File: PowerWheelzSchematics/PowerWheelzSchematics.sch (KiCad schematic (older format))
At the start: 0 parts

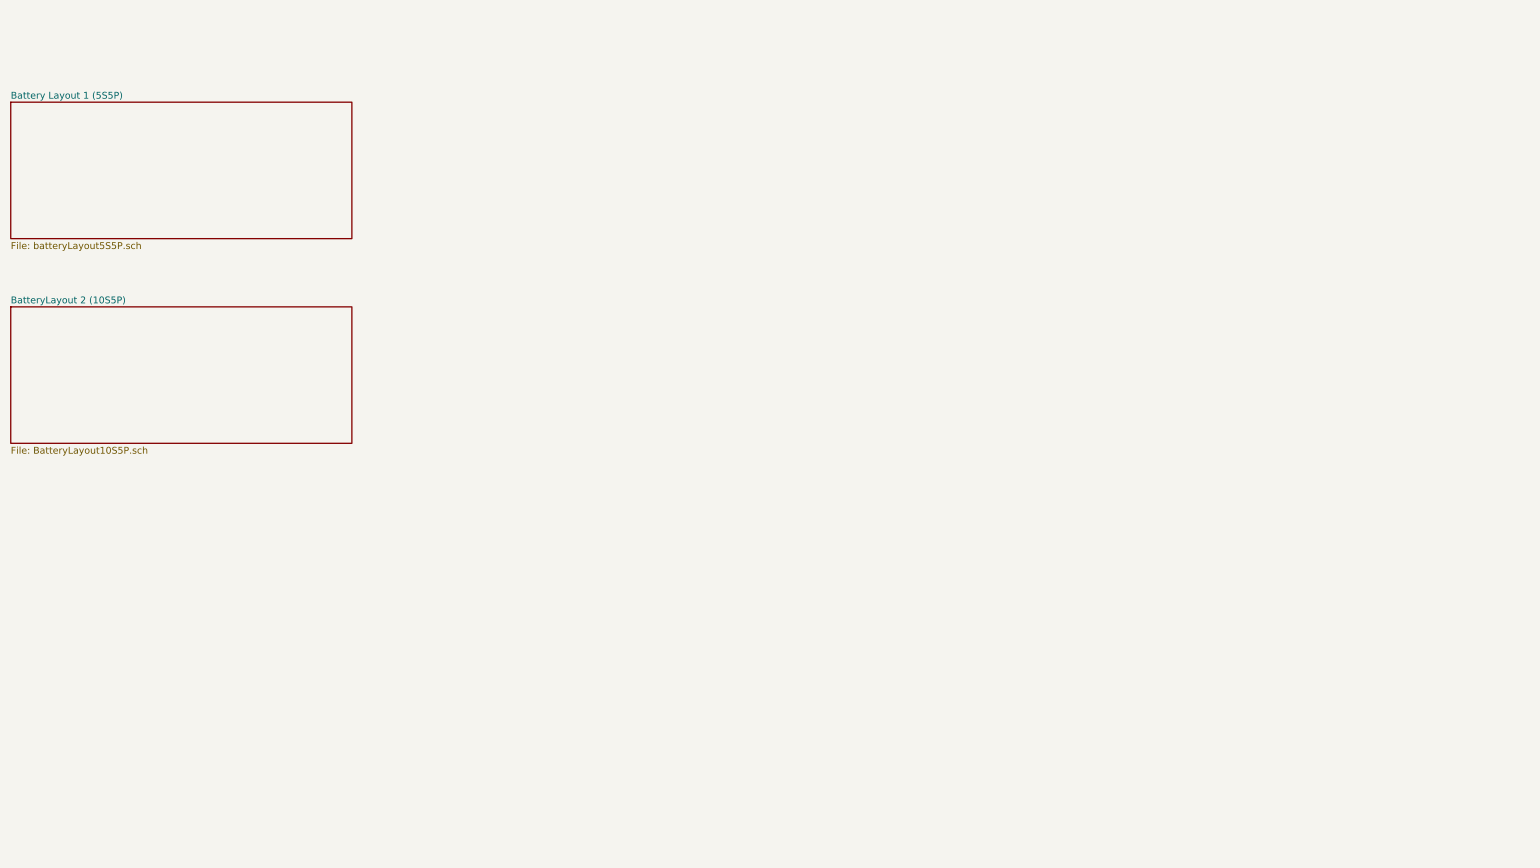
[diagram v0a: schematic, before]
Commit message: Big Update
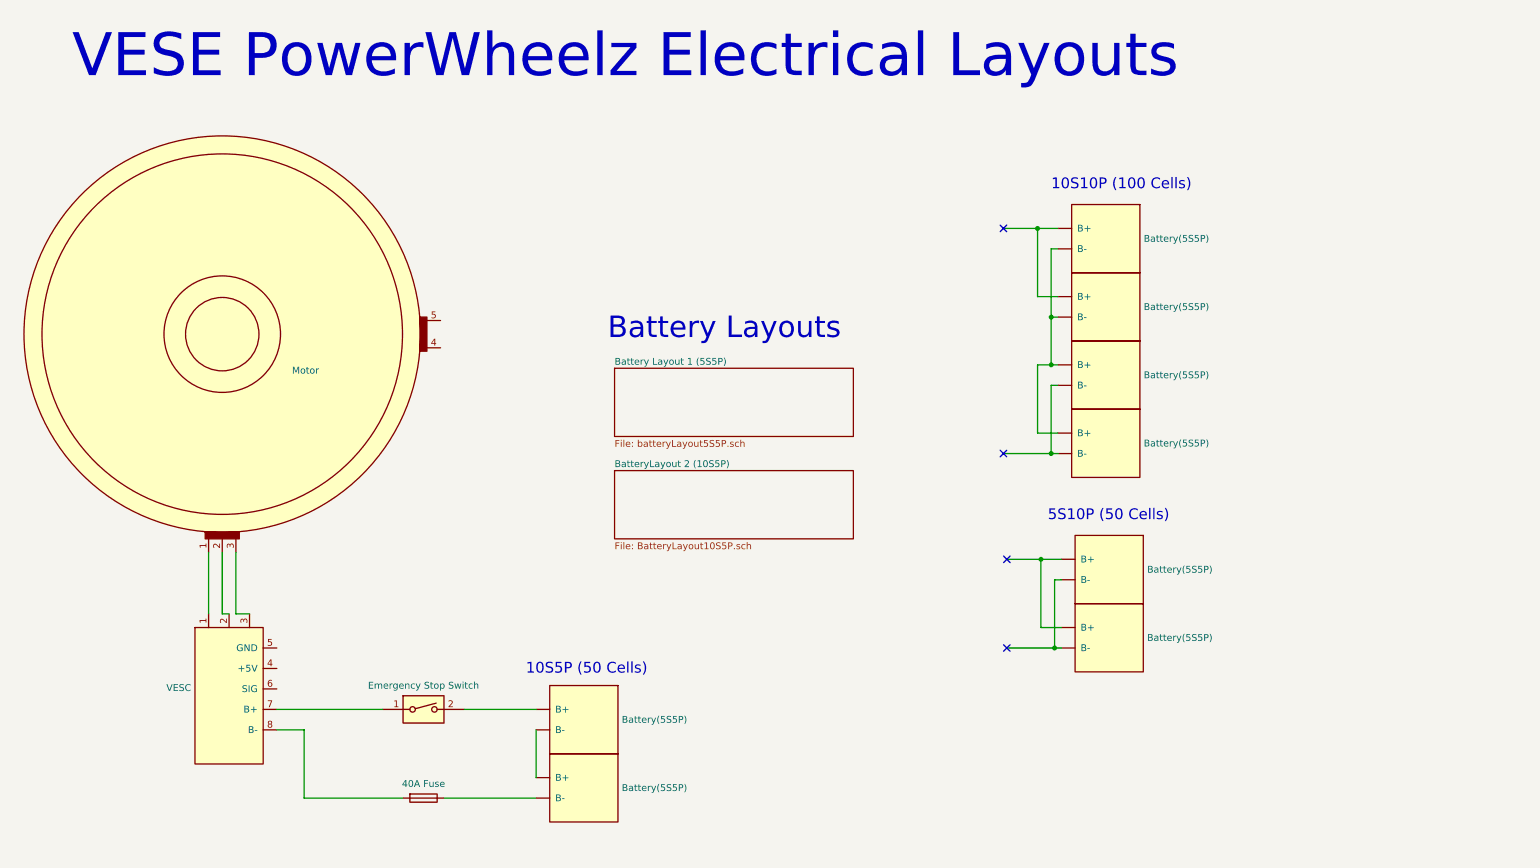
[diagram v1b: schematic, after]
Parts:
- added F: 40A Fuse, symbol Device:Fuse
- added SW?: Emergency Stop Switch, symbol Switch:SW_DIP_x01
- added U?: VESC, symbol VESE:VESC
- added U?: Motor, symbol VESE:Motor
- added U? (x8): Battery(5S5P), symbol VESE:Battery(5S5P)
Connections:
- new net: U?.1, U?.1
- new net: U?.2, U?.2
- new net: U?.3, U?.3
- new net: SW?.1, U?.7 (B+)
- new net: F.2, U?.8 (B-)
- new net: U?.~ (B-), U?.~ (B-) (x5)
- new net: U?.~ (B-), U?.~ (B-), U?.~ (B-), U?.~ (B-)
- new net: SW?.2, U?.~ (B-)
- new net: F.1, U?.~ (B-)
- no-connect marks 0 -> 4
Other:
- note added: "10S10P (100 Cells)"
- note added: "10S5P (50 Cells)"
- note added: "5S10P (50 Cells)"
- note added: "Battery Layouts"
- note added: "VESE PowerWheelz Electrical Layouts\n"
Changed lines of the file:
@@
 $EndDescr
 $Sheet
-S 1000 1250 2500 1000
+S 5425 3950 1750 500
+U 5FA8CE26
+F0 "BatteryLayout 2 (10S5P)" 50
+F1 "BatteryLayout10S5P.sch" 50
+$EndSheet
+Wire Wire Line
+	2600 5000 2550 5000
+Wire Wire Line
+	2650 5000 2750 5000
+$Comp
+L VESE:Motor U?
+U 1 1 5F97A74D
+P 2550 2950
+F 0 "U?" H 2550 2950 50  0001 C CNN
+F 1 "Motor" H 3061 2684 50  0000 L CNN
+F 2 "" H 2550 2950 50  0001 C CNN
+F 3 "" H 2550 2950 50  0001 C CNN
+	1    2550 2950
+	1    0    0    -1
+$EndComp
+$Comp
+L VESE:Battery(5S5P) U?
+U 1 1 5F985BDF
+P 9275 3000
+F 0 "U?" H 9275 3000 50  0001 C CNN
+F 1 "Battery(5S5P)" V 9525 3028 50  0000 L CNN
+F 2 "" H 9275 3000 50  0001 C CNN
+F 3 "" H 9275 3000 50  0001 C CNN
+	1    9275 3000
+	0    1    1    0
+$EndComp
+$Comp
+L VESE:Battery(5S5P) U?
+U 1 1 5F987B8F
+P 9275 3500
+F 0 "U?" H 9275 3500 50  0001 C CNN
+F 1 "Battery(5S5P)" V 9525 3528 50  0000 L CNN
+F 2 "" H 9275 3500 50  0001 C CNN
+F 3 "" H 9275 3500 50  0001 C CNN
+	1    9275 3500
+	0    1    1    0
+$EndComp
+Wire Wire Line
+	4850 5850 4850 6200
+Wire Wire Line
+	3150 5850 2950 5850
+Wire Wire Line
+	3150 6350 3150 5850
+$Comp
+L VESE:VESC U?
+U 1 1 5F96E5B6
+P 2350 5100
+F 0 "U?" H 2350 5100 50  0001 C CNN
+F 1 "VESC" H 2322 4658 50  0000 R CNN
+F 2 "" H 2350 5100 50  0001 C CNN
+F 3 "" H 2350 5100 50  0001 C CNN
+	1    2350 5100
+	1    0    0    -1
+$EndComp
+$Comp
+L Switch:SW_DIP_x01 SW?
+U 1 1 5F9C224C
+P 4025 5700
+F 0 "SW?" H 4025 5967 50  0001 C CNN
+F 1 "Emergency Stop Switch" H 4025 5875 50  0000 C CNN
+F 2 "" H 4025 5700 50  0001 C CNN
+F 3 "~" H 4025 5700 50  0001 C CNN
+	1    4025 5700
+	1    0    0    -1
+$EndComp
+Wire Wire Line
+	3150 6350 3875 6350
+Wire Wire Line
+	2950 5700 3725 5700
+Wire Wire Line
+	4325 5700 4850 5700
+Text Notes 1450 1100 0    315  ~ 0
+VESE PowerWheelz Electrical Layouts\n
+Text Notes 5375 3000 0    157  ~ 0
+Battery Layouts
+$Sheet
+S 5425 3200 1750 500
 U 5F8680B4
 F0 "Battery Layout 1 (5S5P)" 50
 F1 "batteryLayout5S5P.sch" 50
 $EndSheet
-$Sheet
-S 1000 2750 2500 1000
-U 5FA8CE26
-F0 "BatteryLayout 2 (10S5P)" 50
-F1 "BatteryLayout10S5P.sch" 50
-$EndSheet
+Wire Wire Line
+	2450 4550 2450 5000
+Wire Wire Line
+	2550 4550 2550 5000
+Wire Wire Line
+	2650 4550 2650 5000
+$Comp
+L Device:Fuse F
+U 1 1 5F9D666D
+P 4025 6350
+F 0 "F" V 3828 6350 50  0001 C CNN
+F 1 "40A Fuse" V 3920 6350 50  0000 C CNN
+F 2 "" V 3955 6350 50  0001 C CNN
+F 3 "~" H 4025 6350 50  0001 C CNN
+	1    4025 6350
+	0    1    1    0
+$EndComp
+Wire Wire Line
+	4175 6350 4850 6350
+$Comp
+L VESE:Battery(5S5P) U?
+U 1 1 5F9E11C0
+P 9275 2000
+F 0 "U?" H 9275 2000 50  0001 C CNN
+F 1 "Battery(5S5P)" V 9525 2028 50  0000 L CNN
+F 2 "" H 9275 2000 50  0001 C CNN
+F 3 "" H 9275 2000 50  0001 C CNN
+	1    9275 2000
+	0    1    1    0
+$EndComp
+$Comp
+L VESE:Battery(5S5P) U?
+U 1 1 5F9E11C6
+P 9275 2500
+F 0 "U?" H 9275 2500 50  0001 C CNN
+F 1 "Battery(5S5P)" V 9525 2528 50  0000 L CNN
+F 2 "" H 9275 2500 50  0001 C CNN
+F 3 "" H 9275 2500 50  0001 C CNN
+	1    9275 2500
+	0    1    1    0
+$EndComp
+Wire Wire Line
+	8525 2675 8525 2175
+Wire Wire Line
+	8525 2175 8675 2175
+Wire Wire Line
+	8525 2675 8675 2675
+Wire Wire Line
+	8675 2325 8625 2325
+Wire Wire Line
+	8625 2325 8625 2825
+Wire Wire Line
+	8625 2825 8675 2825
+Wire Wire Line
+	8525 3175 8525 3675
+Wire Wire Line
+	8525 3675 8675 3675
+Wire Wire Line
+	8675 3325 8625 3325
+Wire Wire Line
+	8625 3325 8625 3825
+Wire Wire Line
+	8625 3825 8675 3825
+Wire Wire Line
+	8625 3825 8275 3825
+Connection ~ 8625 3825
+Wire Wire Line
+	8525 2175 8275 2175
+Connection ~ 8525 2175
+Wire Wire Line
+	8625 2825 8625 3175
+Wire Wire Line
+	8525 3175 8625 3175
+Connection ~ 8625 2825
+Connection ~ 8625 3175
+Wire Wire Line
+	8625 3175 8675 3175
+$Comp
+L VESE:Battery(5S5P) U?
+U 1 1 5F9F8610
+P 5450 5525
+F 0 "U?" H 5450 5525 50  0001 C CNN
+F 1 "Battery(5S5P)" V 5700 5553 50  0000 L CNN
+F 2 "" H 5450 5525 50  0001 C CNN
+F 3 "" H 5450 5525 50  0001 C CNN
+	1    5450 5525
+	0    1    1    0
+$EndComp
+$Comp
+L VESE:Battery(5S5P) U?
+U 1 1 5F9F8616
+P 5450 6025
+F 0 "U?" H 5450 6025 50  0001 C CNN
+F 1 "Battery(5S5P)" V 5700 6053 50  0000 L CNN
+F 2 "" H 5450 6025 50  0001 C CNN
+F 3 "" H 5450 6025 50  0001 C CNN
+	1    5450 6025
+	0    1    1    0
+$EndComp
+NoConn ~ 8275 3825
+NoConn ~ 8275 2175
+Text Notes 4775 5450 0    79   ~ 0
+10S5P (50 Cells)
+Text Notes 8625 1900 0    79   ~ 0
+10S10P (100 Cells)
+$Comp
+L VESE:Battery(5S5P) U?
+U 1 1 5FA0FAAC
+P 9300 4425
+F 0 "U?" H 9300 4425 50  0001 C CNN
+F 1 "Battery(5S5P)" V 9550 4453 50  0000 L CNN
+F 2 "" H 9300 4425 50  0001 C CNN
+F 3 "" H 9300 4425 50  0001 C CNN
+	1    9300 4425
+	0    1    1    0
+$EndComp
+$Comp
+L VESE:Battery(5S5P) U?
+U 1 1 5FA0FAB2
+P 9300 4925
+F 0 "U?" H 9300 4925 50  0001 C CNN
+F 1 "Battery(5S5P)" V 9550 4953 50  0000 L CNN
+F 2 "" H 9300 4925 50  0001 C CNN
+F 3 "" H 9300 4925 50  0001 C CNN
+	1    9300 4925
+	0    1    1    0
+$EndComp
+Wire Wire Line
+	8700 5100 8550 5100
+Wire Wire Line
+	8550 5100 8550 4600
+Wire Wire Line
+	8550 4600 8700 4600
+Wire Wire Line
+	8700 4750 8650 4750
+Wire Wire Line
+	8650 4750 8650 5250
+Wire Wire Line
+	8650 5250 8700 5250
+Wire Wire Line
+	8550 4600 8300 4600
+Connection ~ 8550 4600
+Wire Wire Line
+	8650 5250 8300 5250
+Connection ~ 8650 5250
+NoConn ~ 8300 4600
+NoConn ~ 8300 5250
+Text Notes 8600 4325 0    79   ~ 0
+5S10P (50 Cells)
 $EndSCHEMATC

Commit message: supply
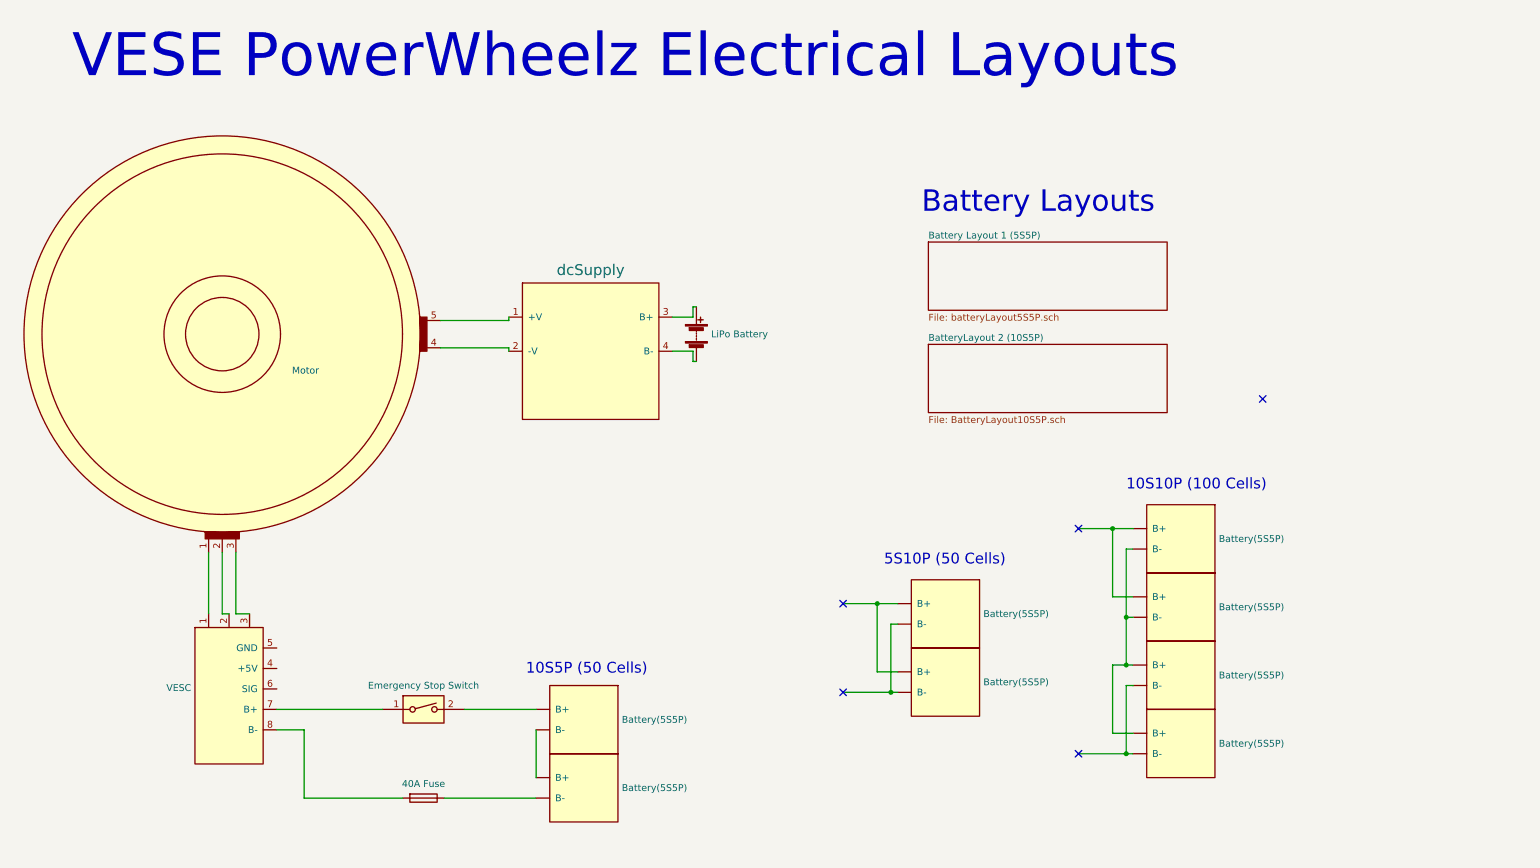
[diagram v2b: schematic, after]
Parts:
- added BT?: LiPo Battery, symbol Device:Battery
- added U?: dcSupply, symbol VESE:dcSupply
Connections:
- net at U?.4: now also U?.2 (-V)
- net at U?.5: now also U?.1 (+V)
- net at U?.~ (B-), U?.~ (B-): now also U?.~ (B-), U?.~ (B-)
- net at U?.~ (B-), U?.~ (B-): no longer U?.~ (B-), U?.~ (B-)
- new net: U?.~ (B-), U?.~ (B-) (x2)
- new net: BT?.1 (+), U?.3 (B+)
- new net: BT?.2 (-), U?.4 (B-)
- no-connect marks 4 -> 5
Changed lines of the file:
@@
 Comment4 ""
 $EndDescr
-$Sheet
-S 5425 3950 1750 500
-U 5FA8CE26
-F0 "BatteryLayout 2 (10S5P)" 50
-F1 "BatteryLayout10S5P.sch" 50
-$EndSheet
 Wire Wire Line
 	2600 5000 2550 5000
@@
 	1    0    0    -1
 $EndComp
-$Comp
-L VESE:Battery(5S5P) U?
-U 1 1 5F985BDF
-P 9275 3000
-F 0 "U?" H 9275 3000 50  0001 C CNN
-F 1 "Battery(5S5P)" V 9525 3028 50  0000 L CNN
-F 2 "" H 9275 3000 50  0001 C CNN
-F 3 "" H 9275 3000 50  0001 C CNN
-	1    9275 3000
-	0    1    1    0
-$EndComp
-$Comp
-L VESE:Battery(5S5P) U?
-U 1 1 5F987B8F
-P 9275 3500
-F 0 "U?" H 9275 3500 50  0001 C CNN
-F 1 "Battery(5S5P)" V 9525 3528 50  0000 L CNN
-F 2 "" H 9275 3500 50  0001 C CNN
-F 3 "" H 9275 3500 50  0001 C CNN
-	1    9275 3500
-	0    1    1    0
-$EndComp
 Wire Wire Line
 	4850 5850 4850 6200
@@
 Text Notes 1450 1100 0    315  ~ 0
 VESE PowerWheelz Electrical Layouts\n
-Text Notes 5375 3000 0    157  ~ 0
+Text Notes 7675 2075 0    157  ~ 0
 Battery Layouts
 $Sheet
-S 5425 3200 1750 500
+S 7725 2275 1750 500
 U 5F8680B4
 F0 "Battery Layout 1 (5S5P)" 50
@@
 $Comp
 L VESE:Battery(5S5P) U?
-U 1 1 5F9E11C0
-P 9275 2000
-F 0 "U?" H 9275 2000 50  0001 C CNN
-F 1 "Battery(5S5P)" V 9525 2028 50  0000 L CNN
-F 2 "" H 9275 2000 50  0001 C CNN
-F 3 "" H 9275 2000 50  0001 C CNN
-	1    9275 2000
-	0    1    1    0
-$EndComp
-$Comp
-L VESE:Battery(5S5P) U?
-U 1 1 5F9E11C6
-P 9275 2500
-F 0 "U?" H 9275 2500 50  0001 C CNN
-F 1 "Battery(5S5P)" V 9525 2528 50  0000 L CNN
-F 2 "" H 9275 2500 50  0001 C CNN
-F 3 "" H 9275 2500 50  0001 C CNN
-	1    9275 2500
-	0    1    1    0
-$EndComp
-Wire Wire Line
-	8525 2675 8525 2175
-Wire Wire Line
-	8525 2175 8675 2175
-Wire Wire Line
-	8525 2675 8675 2675
-Wire Wire Line
-	8675 2325 8625 2325
-Wire Wire Line
-	8625 2325 8625 2825
-Wire Wire Line
-	8625 2825 8675 2825
-Wire Wire Line
-	8525 3175 8525 3675
-Wire Wire Line
-	8525 3675 8675 3675
-Wire Wire Line
-	8675 3325 8625 3325
-Wire Wire Line
-	8625 3325 8625 3825
-Wire Wire Line
-	8625 3825 8675 3825
-Wire Wire Line
-	8625 3825 8275 3825
-Connection ~ 8625 3825
-Wire Wire Line
-	8525 2175 8275 2175
-Connection ~ 8525 2175
-Wire Wire Line
-	8625 2825 8625 3175
-Wire Wire Line
-	8525 3175 8625 3175
-Connection ~ 8625 2825
-Connection ~ 8625 3175
-Wire Wire Line
-	8625 3175 8675 3175
-$Comp
-L VESE:Battery(5S5P) U?
 U 1 1 5F9F8610
 P 5450 5525
@@
 	0    1    1    0
 $EndComp
-NoConn ~ 8275 3825
-NoConn ~ 8275 2175
 Text Notes 4775 5450 0    79   ~ 0
 10S5P (50 Cells)
-Text Notes 8625 1900 0    79   ~ 0
+NoConn ~ 7100 4925
+NoConn ~ 10175 3425
+Wire Wire Line
+	7350 4925 7100 4925
+Wire Wire Line
+	7350 5425 7350 4925
+Connection ~ 7350 4925
+$Comp
+L VESE:Battery(5S5P) U?
+U 1 1 5F985BDF
+P 9825 5200
+F 0 "U?" H 9825 5200 50  0001 C CNN
+F 1 "Battery(5S5P)" V 10075 5228 50  0000 L CNN
+F 2 "" H 9825 5200 50  0001 C CNN
+F 3 "" H 9825 5200 50  0001 C CNN
+	1    9825 5200
+	0    1    1    0
+$EndComp
+$Comp
+L VESE:Battery(5S5P) U?
+U 1 1 5F987B8F
+P 9825 5700
+F 0 "U?" H 9825 5700 50  0001 C CNN
+F 1 "Battery(5S5P)" V 10075 5728 50  0000 L CNN
+F 2 "" H 9825 5700 50  0001 C CNN
+F 3 "" H 9825 5700 50  0001 C CNN
+	1    9825 5700
+	0    1    1    0
+$EndComp
+$Comp
+L VESE:Battery(5S5P) U?
+U 1 1 5F9E11C0
+P 9825 4200
+F 0 "U?" H 9825 4200 50  0001 C CNN
+F 1 "Battery(5S5P)" V 10075 4228 50  0000 L CNN
+F 2 "" H 9825 4200 50  0001 C CNN
+F 3 "" H 9825 4200 50  0001 C CNN
+	1    9825 4200
+	0    1    1    0
+$EndComp
+$Comp
+L VESE:Battery(5S5P) U?
+U 1 1 5F9E11C6
+P 9825 4700
+F 0 "U?" H 9825 4700 50  0001 C CNN
+F 1 "Battery(5S5P)" V 10075 4728 50  0000 L CNN
+F 2 "" H 9825 4700 50  0001 C CNN
+F 3 "" H 9825 4700 50  0001 C CNN
+	1    9825 4700
+	0    1    1    0
+$EndComp
+Wire Wire Line
+	9075 4875 9075 4375
+Wire Wire Line
+	9075 4875 9225 4875
+Wire Wire Line
+	9175 4525 9175 5025
+Wire Wire Line
+	9175 5025 9225 5025
+Wire Wire Line
+	9075 5375 9075 5875
+Wire Wire Line
+	9075 5875 9225 5875
+Wire Wire Line
+	9225 5525 9175 5525
+Wire Wire Line
+	9175 5525 9175 6025
+Wire Wire Line
+	9175 6025 9225 6025
+Wire Wire Line
+	9175 6025 8825 6025
+Connection ~ 9175 6025
+Wire Wire Line
+	9175 5025 9175 5375
+Wire Wire Line
+	9075 5375 9175 5375
+Connection ~ 9175 5025
+Connection ~ 9175 5375
+Wire Wire Line
+	9175 5375 9225 5375
+NoConn ~ 8825 6025
+$Comp
+L VESE:Battery(5S5P) U?
+U 1 1 5FA0FAAC
+P 8100 4750
+F 0 "U?" H 8100 4750 50  0001 C CNN
+F 1 "Battery(5S5P)" V 8350 4778 50  0000 L CNN
+F 2 "" H 8100 4750 50  0001 C CNN
+F 3 "" H 8100 4750 50  0001 C CNN
+	1    8100 4750
+	0    1    1    0
+$EndComp
+$Comp
+L VESE:Battery(5S5P) U?
+U 1 1 5FA0FAB2
+P 8100 5250
+F 0 "U?" H 8100 5250 50  0001 C CNN
+F 1 "Battery(5S5P)" V 8350 5278 50  0000 L CNN
+F 2 "" H 8100 5250 50  0001 C CNN
+F 3 "" H 8100 5250 50  0001 C CNN
+	1    8100 5250
+	0    1    1    0
+$EndComp
+Wire Wire Line
+	7500 5425 7350 5425
+Wire Wire Line
+	7350 4925 7500 4925
+Wire Wire Line
+	7500 5075 7450 5075
+Wire Wire Line
+	7450 5075 7450 5575
+Wire Wire Line
+	7450 5575 7500 5575
+Wire Wire Line
+	7450 5575 7100 5575
+Connection ~ 7450 5575
+Text Notes 7400 4650 0    79   ~ 0
+5S10P (50 Cells)
+Wire Wire Line
+	9075 4375 9225 4375
+Wire Wire Line
+	9075 4375 8825 4375
+Connection ~ 9075 4375
+NoConn ~ 8825 4375
+Wire Wire Line
+	9225 4525 9175 4525
+NoConn ~ 7100 5575
+$Comp
+L VESE:dcSupply U?
+U 1 1 5FA45B1A
+P 4750 2575
+F 0 "U?" H 4750 2575 79  0001 C CNN
+F 1 "dcSupply" H 5250 2670 79  0000 C CNN
+F 2 "" H 4750 2575 79  0001 C CNN
+F 3 "" H 4750 2575 79  0001 C CNN
+	1    4750 2575
+	1    0    0    -1
+$EndComp
+Wire Wire Line
+	4150 3050 4650 3050
+Wire Wire Line
+	4650 3050 4650 3075
+Wire Wire Line
+	4150 2850 4650 2850
+Wire Wire Line
+	4650 2850 4650 2825
+$Comp
+L Device:Battery BT?
+U 1 1 5FA49CBC
+P 6025 2950
+F 0 "BT?" H 6133 2996 50  0001 L CNN
+F 1 "LiPo Battery" H 6133 2950 50  0000 L CNN
+F 2 "" V 6025 3010 50  0001 C CNN
+F 3 "~" V 6025 3010 50  0001 C CNN
+	1    6025 2950
+	1    0    0    -1
+$EndComp
+Wire Wire Line
+	5850 3075 6000 3075
+Wire Wire Line
+	6000 3075 6000 3150
+Wire Wire Line
+	6000 3150 6025 3150
+Wire Wire Line
+	5850 2825 6000 2825
+Wire Wire Line
+	6000 2825 6000 2750
+Wire Wire Line
+	6000 2750 6025 2750
+Text Notes 9175 4100 0    79   ~ 0
 10S10P (100 Cells)
-$Comp
-L VESE:Battery(5S5P) U?
-U 1 1 5FA0FAAC
-P 9300 4425
-F 0 "U?" H 9300 4425 50  0001 C CNN
-F 1 "Battery(5S5P)" V 9550 4453 50  0000 L CNN
-F 2 "" H 9300 4425 50  0001 C CNN
-F 3 "" H 9300 4425 50  0001 C CNN
-	1    9300 4425
-	0    1    1    0
-$EndComp
-$Comp
-L VESE:Battery(5S5P) U?
-U 1 1 5FA0FAB2
-P 9300 4925
-F 0 "U?" H 9300 4925 50  0001 C CNN
-F 1 "Battery(5S5P)" V 9550 4953 50  0000 L CNN
-F 2 "" H 9300 4925 50  0001 C CNN
-F 3 "" H 9300 4925 50  0001 C CNN
-	1    9300 4925
-	0    1    1    0
-$EndComp
-Wire Wire Line
-	8700 5100 8550 5100
-Wire Wire Line
-	8550 5100 8550 4600
-Wire Wire Line
-	8550 4600 8700 4600
-Wire Wire Line
-	8700 4750 8650 4750
-Wire Wire Line
-	8650 4750 8650 5250
-Wire Wire Line
-	8650 5250 8700 5250
-Wire Wire Line
-	8550 4600 8300 4600
-Connection ~ 8550 4600
-Wire Wire Line
-	8650 5250 8300 5250
-Connection ~ 8650 5250
-NoConn ~ 8300 4600
-NoConn ~ 8300 5250
-Text Notes 8600 4325 0    79   ~ 0
-5S10P (50 Cells)
+$Sheet
+S 7725 3025 1750 500
+U 5FA8CE26
+F0 "BatteryLayout 2 (10S5P)" 50
+F1 "BatteryLayout10S5P.sch" 50
+$EndSheet
 $EndSCHEMATC
